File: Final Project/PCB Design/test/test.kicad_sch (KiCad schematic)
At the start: 56 parts, among them J1 Motor_Input_1, J10 LED_Out_2, J11 PSoC_SDA, J12 PSoC_SCL, J13 LCD_VCC, J14 LCD_GND, J15 LCD_SDA, J16 LCD_SCL, J17 RTC_VCC, J18 RTC_GND, J19 RTC_SDA, J2 Motor_Input_2, J20 RTC_SCL, J21 LED_Out_3, J22 LED_Out_4, J23 LED_In_1, J24 LED_In_2, J25 LED_In_3, J26 LED_In_4, J27 LED_GND_1, J28 LED_GND_2, J29 LED_GND_3, J3 Motor_Input_3, J30 LED_GND_4, J31 Speaker_1_PWR, J32 Speaker_1_PWR, J33 Speaker_1_GND, J34 Speaker_2_GND, J35 Speaker_GPIO, J36 RTC_INT, J37 RTC_COT, J38 PSoC_RTC_INT, J39 PSoC_RTC_COT, J4 Motor_Input_4, J40 BTN_IN, J41 BTN_OUT, J42 PSoC_BTN_OUT, J5 13.5V, J6 13.5V GND, J7 5V, J8 5V GND, J9 LED_Out_1, M1 Stepper_Motor_bipolar, Q1 PN2222A, Q2 PN2222A, U1 L293D

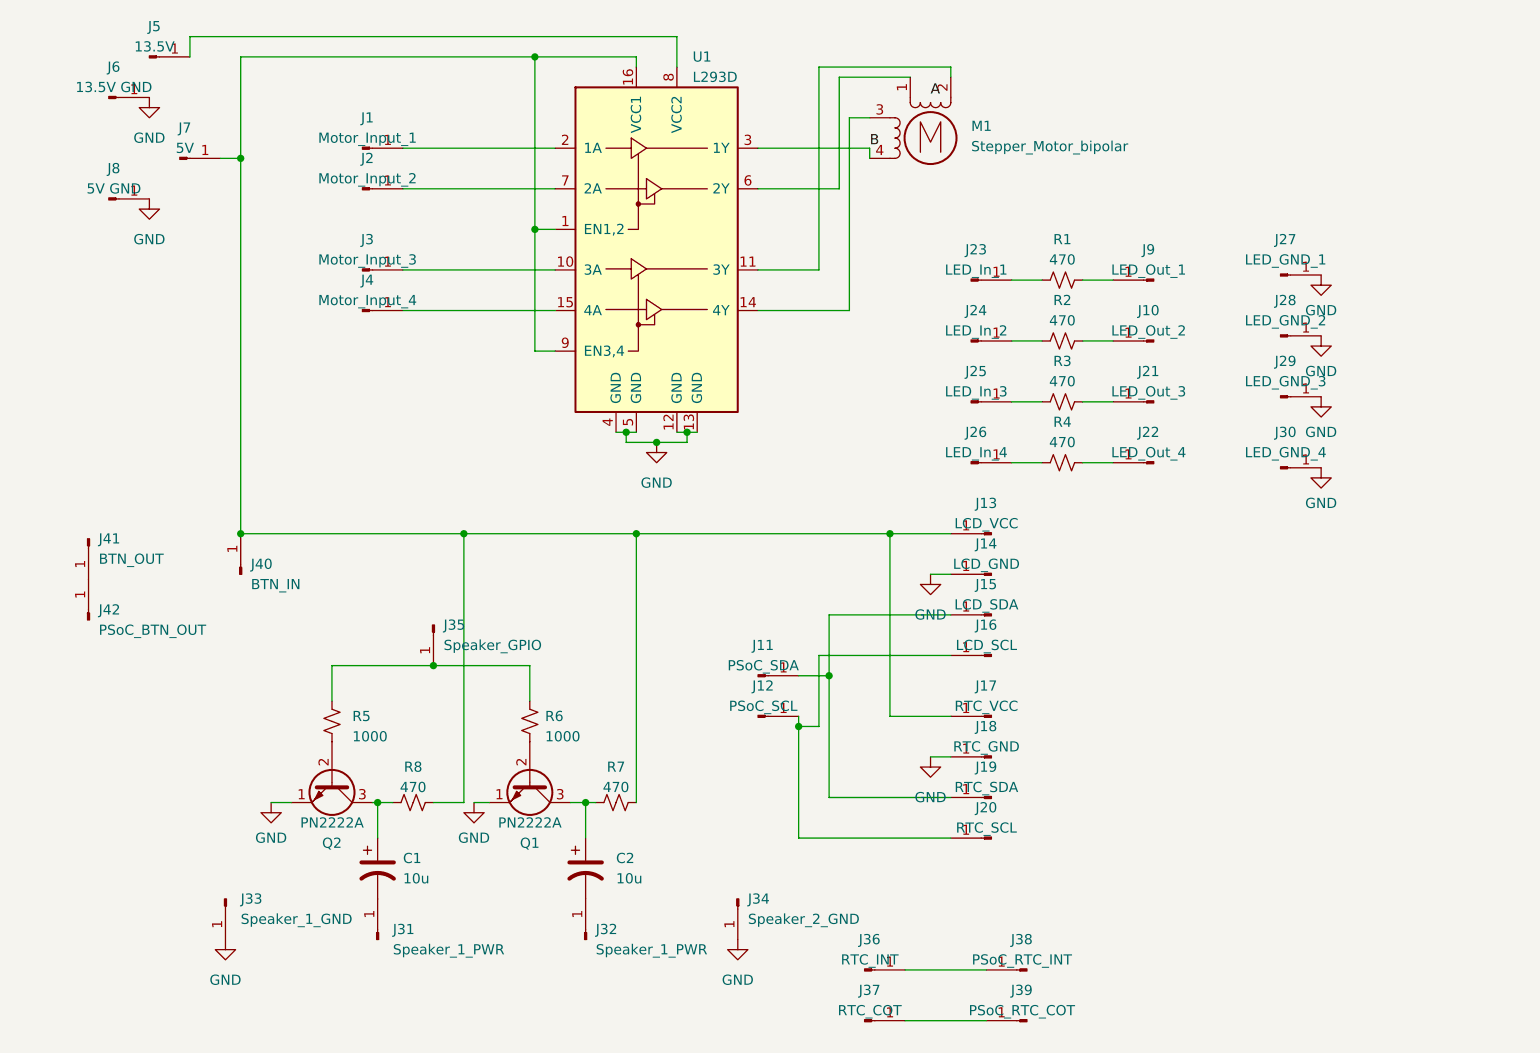
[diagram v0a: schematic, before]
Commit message: Edited pcb
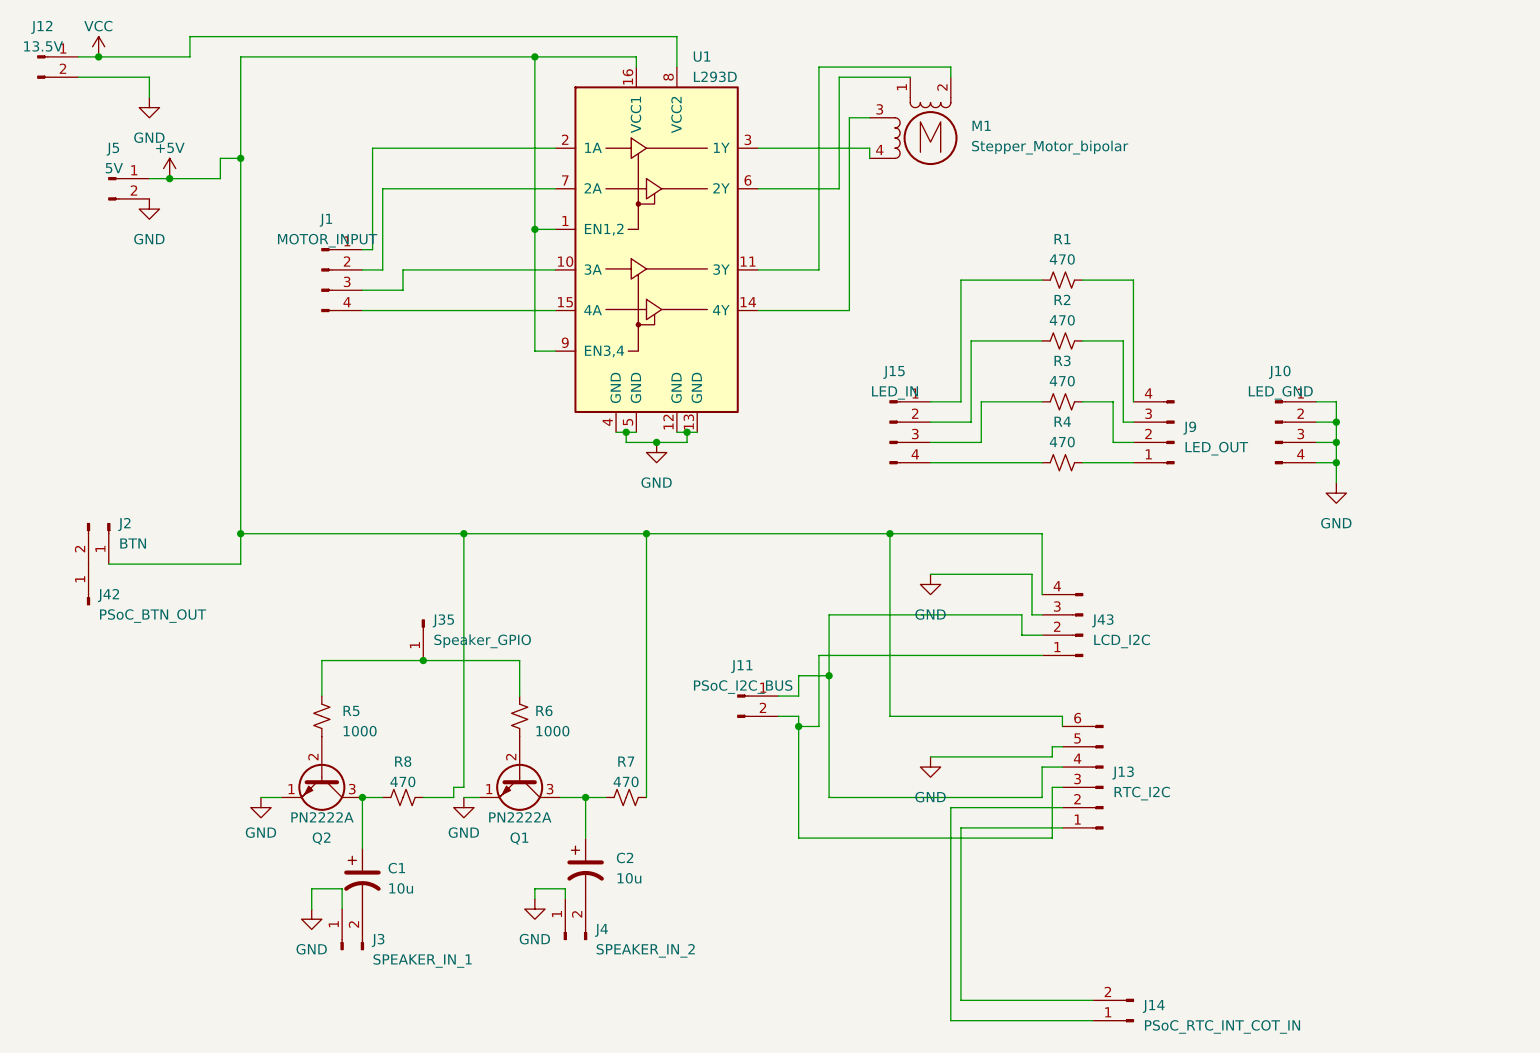
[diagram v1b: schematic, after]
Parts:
- removed J1: Motor_Input_1, symbol Connector:Conn_01x01_Pin
- removed J10: LED_Out_2, symbol Connector:Conn_01x01_Pin
- removed J11: PSoC_SDA, symbol Connector:Conn_01x01_Pin
- removed J12: PSoC_SCL, symbol Connector:Conn_01x01_Pin
- removed J13: LCD_VCC, symbol Connector:Conn_01x01_Pin
- removed J14: LCD_GND, symbol Connector:Conn_01x01_Pin
- removed J15: LCD_SDA, symbol Connector:Conn_01x01_Pin
- removed J16: LCD_SCL, symbol Connector:Conn_01x01_Pin
- removed J17: RTC_VCC, symbol Connector:Conn_01x01_Pin
- removed J18: RTC_GND, symbol Connector:Conn_01x01_Pin
- removed J19: RTC_SDA, symbol Connector:Conn_01x01_Pin
- removed J2: Motor_Input_2, symbol Connector:Conn_01x01_Pin
- removed J20: RTC_SCL, symbol Connector:Conn_01x01_Pin
- removed J21: LED_Out_3, symbol Connector:Conn_01x01_Pin
- removed J22: LED_Out_4, symbol Connector:Conn_01x01_Pin
- removed J23: LED_In_1, symbol Connector:Conn_01x01_Pin
- removed J24: LED_In_2, symbol Connector:Conn_01x01_Pin
- removed J25: LED_In_3, symbol Connector:Conn_01x01_Pin
- removed J26: LED_In_4, symbol Connector:Conn_01x01_Pin
- removed J27: LED_GND_1, symbol Connector:Conn_01x01_Pin
- removed J28: LED_GND_2, symbol Connector:Conn_01x01_Pin
- removed J29: LED_GND_3, symbol Connector:Conn_01x01_Pin
- removed J3: Motor_Input_3, symbol Connector:Conn_01x01_Pin
- removed J30: LED_GND_4, symbol Connector:Conn_01x01_Pin
- removed J31, J32: Speaker_1_PWR, symbol Connector:Conn_01x01_Pin
- removed J33: Speaker_1_GND, symbol Connector:Conn_01x01_Pin
- removed J34: Speaker_2_GND, symbol Connector:Conn_01x01_Pin
- removed J36: RTC_INT, symbol Connector:Conn_01x01_Pin
- removed J37: RTC_COT, symbol Connector:Conn_01x01_Pin
- removed J38: PSoC_RTC_INT, symbol Connector:Conn_01x01_Pin
- removed J39: PSoC_RTC_COT, symbol Connector:Conn_01x01_Pin
- removed J4: Motor_Input_4, symbol Connector:Conn_01x01_Pin
- removed J40: BTN_IN, symbol Connector:Conn_01x01_Pin
- removed J41: BTN_OUT, symbol Connector:Conn_01x01_Pin
- removed J5: 13.5V, symbol Connector:Conn_01x01_Pin
- removed J6: 13.5V GND, symbol Connector:Conn_01x01_Pin
- removed J7: 5V, symbol Connector:Conn_01x01_Pin
- removed J8: 5V GND, symbol Connector:Conn_01x01_Pin
- removed J9: LED_Out_1, symbol Connector:Conn_01x01_Pin
- added J1: MOTOR_INPUT, Connector_PinSocket_2.54mm:PinSocket_1x04_P2.54mm_Vertical, symbol Connector:Conn_01x04_Pin
- added J10: LED_GND, Connector_PinSocket_2.54mm:PinSocket_1x04_P2.54mm_Vertical, symbol Connector:Conn_01x04_Pin
- added J11: PSoC_I2C_BUS, Connector_PinHeader_2.54mm:PinHeader_1x02_P2.54mm_Vertical, symbol Connector:Conn_01x02_Pin
- added J12: 13.5V, Connector_PinHeader_2.54mm:PinHeader_1x02_P2.54mm_Vertical, symbol Connector:Conn_01x02_Pin
- added J13: RTC_I2C, Connector_PinHeader_2.54mm:PinHeader_1x06_P2.54mm_Vertical, symbol Connector:Conn_01x06_Pin
- added J14: PSoC_RTC_INT_COT_IN, Connector_PinHeader_2.54mm:PinHeader_1x02_P2.54mm_Vertical, symbol Connector:Conn_01x02_Pin
- added J15: LED_IN, Connector_PinHeader_2.54mm:PinHeader_1x04_P2.54mm_Vertical, symbol Connector:Conn_01x04_Pin
- added J2: BTN, Connector_PinHeader_2.54mm:PinHeader_1x02_P2.54mm_Vertical, symbol Connector:Conn_01x02_Pin
- added J3: SPEAKER_IN_1, Connector_PinHeader_2.54mm:PinHeader_1x02_P2.54mm_Vertical, symbol Connector:Conn_01x02_Pin
- added J4: SPEAKER_IN_2, Connector_PinHeader_2.54mm:PinHeader_1x02_P2.54mm_Vertical, symbol Connector:Conn_01x02_Pin
- added J43: LCD_I2C, Connector_PinSocket_2.54mm:PinSocket_1x04_P2.54mm_Vertical, symbol Connector:Conn_01x04_Pin
- added J5: 5V, Connector_PinHeader_2.54mm:PinHeader_1x02_P2.54mm_Vertical, symbol Connector:Conn_01x02_Pin
- added J9: LED_OUT, Connector_PinSocket_2.54mm:PinSocket_1x04_P2.54mm_Vertical, symbol Connector:Conn_01x04_Pin
- C1, C2: footprint (none) -> Capacitor_THT:CP_Radial_D10.0mm_P7.50mm
- J35, J42: footprint (none) -> Connector_PinHeader_2.54mm:PinHeader_1x01_P2.54mm_Vertical
- M1: footprint (none) -> Connector_PinSocket_2.54mm:PinSocket_1x04_P2.54mm_Vertical
- Q1, Q2: footprint Package_TO_SOT_THT:TO-92_Inline -> Connector_PinHeader_2.54mm:PinHeader_1x03_P2.54mm_Vertical
- R1, R2, R3, R4, R5, R6, R7, R8: footprint (none) -> Resistor_THT:R_Axial_DIN0411_L9.9mm_D3.6mm_P12.70mm_Horizontal
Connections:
- net GND: now also J10.1 (Pin_1), J10.2 (Pin_2), J10.3 (Pin_3), J10.4 (Pin_4), J12.2 (Pin_2), J13.5 (Pin_5), J3.1 (Pin_1), J4.1 (Pin_1), J43.3 (Pin_3), J5.2 (Pin_2)
- net at R1.1: now also J15.1 (Pin_1)
- net at R4.1: now also J15.4 (Pin_4)
- net +5V: now reaches R7.2, R8.2, U1.1 (EN1,2), U1.16 (VCC1), U1.9 (EN3,4)
- net +5V: now also J13.6 (Pin_6), J2.1 (Pin_1), J43.4 (Pin_4), J5.1 (Pin_1)
- net at U1.10 (3A): now also J1.3 (Pin_3)
- net at U1.15 (4A): now also J1.4 (Pin_4)
- net at U1.2 (1A): now also J1.1 (Pin_1)
- net at U1.7 (2A): now also J1.2 (Pin_2)
- net VCC: now reaches U1.8 (VCC2)
- net VCC: now also J12.1 (Pin_1)
- net at C1.2: now also J3.2 (Pin_2)
- net at R1.2: now also J9.4 (Pin_4)
- net at R2.1: now also J15.2 (Pin_2)
- net at R2.2: now also J9.3 (Pin_3)
- net at C2.2: now also J4.2 (Pin_2)
- net at J42.1 (Pin_1): now also J2.2 (Pin_2)
- net at R4.2: now also J9.1 (Pin_1)
- net at R3.1: now also J15.3 (Pin_3)
- net at R3.2: now also J9.2 (Pin_2)
- net B: no longer names the net of M1.4, U1.3 (1Y)
- new net: J13.2 (Pin_2), J14.1 (Pin_1)
- new net: J13.1 (Pin_1), J14.2 (Pin_2)
- new net: J11.1 (Pin_1), J13.4 (Pin_4), J43.2 (Pin_2)
- new net: J11.2 (Pin_2), J13.3 (Pin_3), J43.1 (Pin_1)
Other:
- moved on the sheet: C1, J35, J42, Q1, Q2, R5, R6, R7, R8

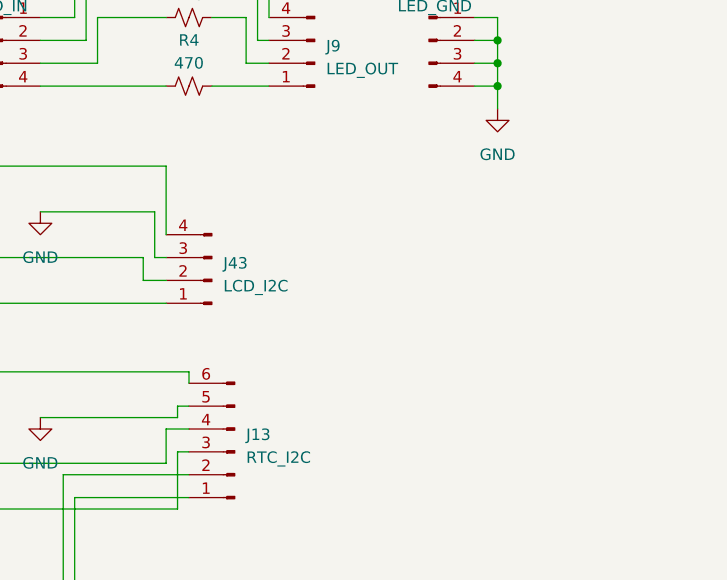
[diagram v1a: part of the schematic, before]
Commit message: final 3D model design and PCB design
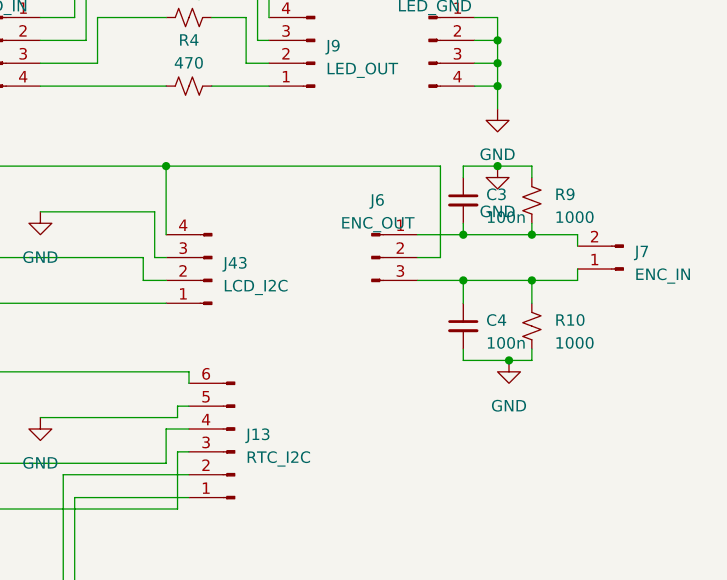
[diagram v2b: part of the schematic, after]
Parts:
- added C3, C4: 100n, Capacitor_THT:C_Disc_D7.5mm_W5.0mm_P5.00mm, symbol Device:C_Small
- added J6: ENC_OUT, Connector_PinHeader_2.54mm:PinHeader_1x03_P2.54mm_Vertical, symbol Connector:Conn_01x03_Pin
- added J7: ENC_IN, Connector_PinHeader_2.54mm:PinHeader_1x02_P2.54mm_Vertical, symbol Connector:Conn_01x02_Pin
- added R10, R9: 1000, Resistor_THT:R_Axial_DIN0411_L9.9mm_D3.6mm_P12.70mm_Horizontal, symbol Device:R_Small_US
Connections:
- net +5V: now also J6.2 (Pin_2)
- net GND: now also C3.1, C4.2, R10.1, R9.2
- new net: C3.2, J6.1 (Pin_1), J7.2 (Pin_2), R9.1
- new net: C4.1, J6.3 (Pin_3), J7.1 (Pin_1), R10.2
